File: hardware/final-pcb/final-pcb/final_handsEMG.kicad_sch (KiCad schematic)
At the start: 190 parts, among them J1 Conn_02x13_Odd_Even, U1 ADS1299CPAG, U2 STM32L496ZGT6, U3 LTC3586EUFE-3-PBF, U4 FT231XQ-R, U6 TPS60403DBVT, U8 TPS72325DBVT, U9 TPS73225DBVT

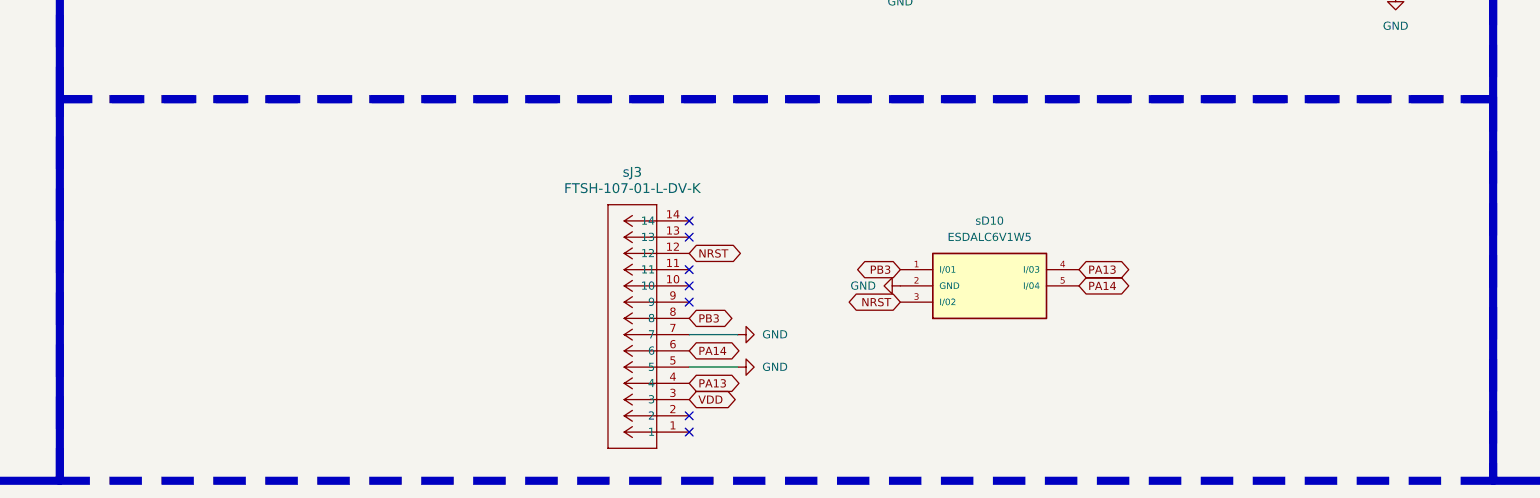
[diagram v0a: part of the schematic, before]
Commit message: lol forgot buttons (4.16.25)
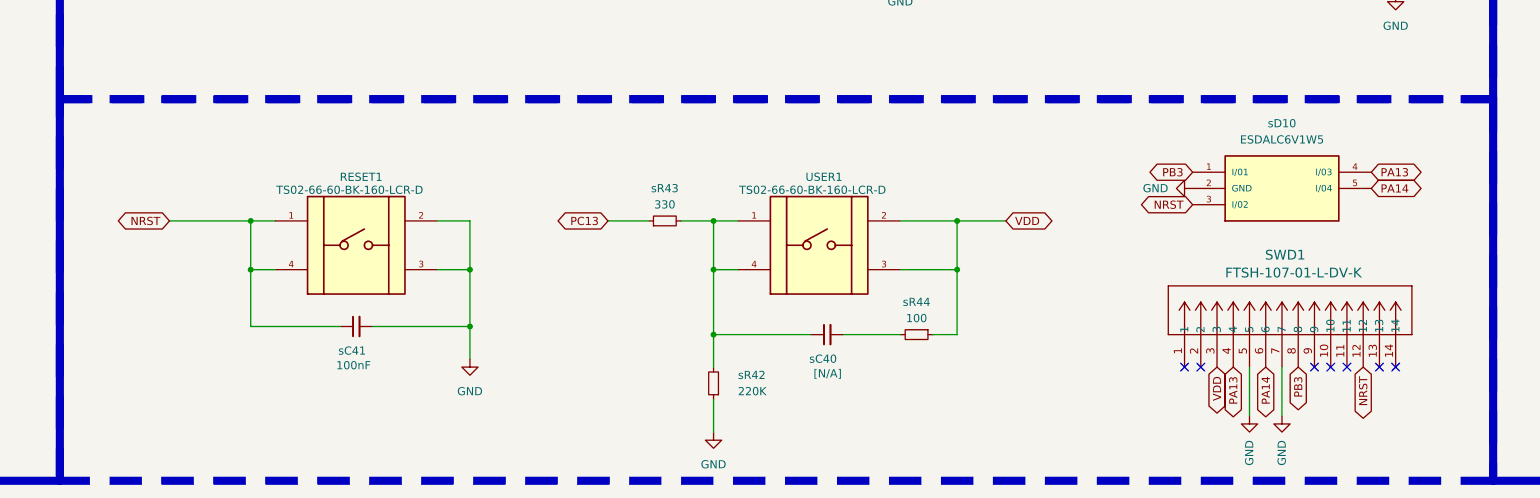
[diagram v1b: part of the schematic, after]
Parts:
- added RESET1, USER1: TS02-66-60-BK-160-LCR-D, FSM6JSMATR:SW_5-1437565-0, symbol TS02-66-60-BK-160-LCR-D:TS02-66-60-BK-160-LCR-D
- added sC40: [N/A], CC0402KRX7R7BB104:YAG_CC0402_YAG, symbol Device:C_Small
- added sC41: 100nF, CC0402KRX7R7BB104:YAG_CC0402_YAG, symbol Device:C_Small
- added sR42: 220K, RC0603FR-07220KL:RESC1607X60N, symbol Device:R_Small
- added sR43: 330, RC0603FR-07330RL:RESC1607X60N, symbol Device:R_Small
- added sR44: 100, RC0603FR-07100RL:RESC1607X60N, symbol Device:R_Small
- renumbered sJ3 to SWD1
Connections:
- net +3V3: now also USER1.2, USER1.3, sR44.1
- net GND: now also RESET1.2, RESET1.3, sC41.2, sR42.1
- net NRST: now also RESET1.1, RESET1.4, sC41.1
- net PC13: now also sR43.1
- new net: USER1.1, USER1.4, sC40.1, sR42.2, sR43.2
- new net: sC40.2, sR44.2
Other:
- moved on the sheet: SWD1, sD10
